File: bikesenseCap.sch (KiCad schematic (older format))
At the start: 43 parts

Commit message: Routing updated
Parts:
- removed D? (x4): LED_Small, symbol Device:LED_Small
- removed J? (x4): PAD, symbol cap1188:PAD
- removed R? (x4): 470, symbol Device:R_Small
- added D11: West, LEDs:LED_0805_HandSoldering, symbol Device:LED_Small
- added D12: NorthWest, LEDs:LED_0805_HandSoldering, symbol Device:LED_Small
- added D13: SouthWest, LEDs:LED_0805_HandSoldering, symbol Device:LED_Small
- added D14: North, LEDs:LED_0805_HandSoldering, symbol Device:LED_Small
- added D15: South, LEDs:LED_0805_HandSoldering, symbol Device:LED_Small
- added D16: NorthEast, LEDs:LED_0805_HandSoldering, symbol Device:LED_Small
- added D17: SouthEast, LEDs:LED_0805_HandSoldering, symbol Device:LED_Small
- added D18: East, LEDs:LED_0805_HandSoldering, symbol Device:LED_Small
- added R19, R21, R22, R27, R28, R31, R32, R35: 66, Resistors_SMD:R_0603_HandSoldering, symbol Device:R_Small
- added R20, R24, R25, R29, R30, R33, R34, R36: 100k, Resistors_SMD:R_0603_HandSoldering, symbol Device:R_Small
- added R23, R26: 10K, Resistors_SMD:R_0603_HandSoldering, symbol Device:R_Small
- added U3: TCA9534, digikey-footprints:SOIC-16_W7.5mm, symbol Interface_Expansion:TCA9534
- D1, D2: renamed from D?; footprint Diode_THT:D_DO-35_SOD27_P7.62mm_Horizontal -> Diodes_SMD:D_SOD-123
- D3, D4, D5, D6: renamed from D?; footprint (none) -> LEDs:LED_0603_HandSoldering
- J1: renamed from J?; footprint (none) -> SeeedOPL-Connector-2016:HW4-2.0
- J10, J11: renamed from J?; footprint (none) -> Connectors:1X01
- J2, J3, J4, J5: renamed from J?; footprint (none) -> capSensingStuff:SensePad
- JP1: renamed from JP?; footprint (none) -> Jumpers:SMT-JUMPER_2_NO_SILK
- R1, R10, R11, R12, R13, R14, R2, R3, R4, R5, R6, R7, R8, R9: renamed from R?; footprint (none) -> Resistors_SMD:R_0603_HandSoldering
- TH1: renamed from TH?; footprint (none) -> Resistors_SMD:R_0603_HandSoldering
- U1: renamed from U?; footprint (none) -> digikey-footprints:VOC_Sensor_LGA-10-1EP-2.7x4mm_CCS811B
- U2: renamed from U?; footprint (none) -> Housings_DFN_QFN:QFN-24_4x4mm_Pitch0.5mm_NoMask
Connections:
- net labels added: East, North, NorthEast, NorthWest, South, SouthEast, SouthWest, West
- wire segments 104 -> 192
- no-connect marks 3 -> 12
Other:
- note added: "CAP1188 - Cap Sensing Controller"
- note added: "CSS811 - VOC Sensor"
- note added: "I2C Connector"
- note added: "LED Interface"
- note added: "Power Flags"
- note added: "TCA9534 - IO Extender"

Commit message: up to revB
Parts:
- D11, D12, D13, D14, D15, D16, D17, D18: footprint LEDs:LED_0805_HandSoldering -> revLed:LED_1206_3216Metric_ReverseMount_Hole1.8x2.4mm
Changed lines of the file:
@@
 F 0 "D18" V 8646 2182 50  0000 R CNN
 F 1 "East" V 8555 2182 50  0000 R CNN
-F 2 "LEDs:LED_0805_HandSoldering" V 8600 2250 50  0001 C CNN
+F 2 "revLed:LED_1206_3216Metric_ReverseMount_Hole1.8x2.4mm" V 8600 2250 50  0001 C CNN
 F 3 "~" V 8600 2250 50  0001 C CNN
 	1    8600 2250
@@
 F 0 "D14" V 7525 1275 50  0000 R CNN
 F 1 "North" V 7425 1325 50  0000 R CNN
-F 2 "LEDs:LED_0805_HandSoldering" V 7500 1350 50  0001 C CNN
+F 2 "revLed:LED_1206_3216Metric_ReverseMount_Hole1.8x2.4mm" V 7500 1350 50  0001 C CNN
 F 3 "~" V 7500 1350 50  0001 C CNN
 	1    7500 1350
@@
 F 0 "D16" V 8146 1707 50  0000 R CNN
 F 1 "NorthEast" V 8055 1707 50  0000 R CNN
-F 2 "LEDs:LED_0805_HandSoldering" V 8100 1775 50  0001 C CNN
+F 2 "revLed:LED_1206_3216Metric_ReverseMount_Hole1.8x2.4mm" V 8100 1775 50  0001 C CNN
 F 3 "~" V 8100 1775 50  0001 C CNN
 	1    8100 1775
@@
 F 0 "D17" V 8146 2707 50  0000 R CNN
 F 1 "SouthEast" V 8055 2707 50  0000 R CNN
-F 2 "LEDs:LED_0805_HandSoldering" V 8100 2775 50  0001 C CNN
+F 2 "revLed:LED_1206_3216Metric_ReverseMount_Hole1.8x2.4mm" V 8100 2775 50  0001 C CNN
 F 3 "~" V 8100 2775 50  0001 C CNN
 	1    8100 2775
@@
 F 0 "D15" V 7546 3082 50  0000 R CNN
 F 1 "South" V 7455 3082 50  0000 R CNN
-F 2 "LEDs:LED_0805_HandSoldering" V 7500 3150 50  0001 C CNN
+F 2 "revLed:LED_1206_3216Metric_ReverseMount_Hole1.8x2.4mm" V 7500 3150 50  0001 C CNN
 F 3 "~" V 7500 3150 50  0001 C CNN
 	1    7500 3150
@@
 F 0 "D13" V 6996 2732 50  0000 R CNN
 F 1 "SouthWest" V 6875 2775 50  0000 R CNN
-F 2 "LEDs:LED_0805_HandSoldering" V 6950 2800 50  0001 C CNN
+F 2 "revLed:LED_1206_3216Metric_ReverseMount_Hole1.8x2.4mm" V 6950 2800 50  0001 C CNN
 F 3 "~" V 6950 2800 50  0001 C CNN
 	1    6950 2800
@@
 F 0 "D11" V 6471 2257 50  0000 R CNN
 F 1 "West" V 6380 2257 50  0000 R CNN
-F 2 "LEDs:LED_0805_HandSoldering" V 6425 2325 50  0001 C CNN
+F 2 "revLed:LED_1206_3216Metric_ReverseMount_Hole1.8x2.4mm" V 6425 2325 50  0001 C CNN
 F 3 "~" V 6425 2325 50  0001 C CNN
 	1    6425 2325
@@
 F 0 "D12" V 6996 1682 50  0000 R CNN
 F 1 "NorthWest" V 6875 1750 50  0000 R CNN
-F 2 "LEDs:LED_0805_HandSoldering" V 6950 1750 50  0001 C CNN
+F 2 "revLed:LED_1206_3216Metric_ReverseMount_Hole1.8x2.4mm" V 6950 1750 50  0001 C CNN
 F 3 "~" V 6950 1750 50  0001 C CNN
 	1    6950 1750

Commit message: REV C
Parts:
- removed D1, D2: 1N4148, Diodes_SMD:D_SOD-123, symbol Diode:1N4148
- removed J10, J11: Conn_01x01, Connectors:1X01, symbol Connector_Generic:Conn_01x01
- removed JP1: SolderJumper_2_Bridged, Jumpers:SMT-JUMPER_2_NO_SILK, symbol Jumper:SolderJumper_2_Bridged
- removed R9: 100K, Resistors_SMD:R_0603_HandSoldering, symbol Device:R_Small
- added R9: 10K, Resistors_SMD:R_0603_HandSoldering, symbol bikesenseCap-rescue:R_Small-Device
- D11, D12, D13, D14, D15, D16, D17, D18, D3, D4, D5, D6: symbol Device:LED_Small -> bikesenseCap-rescue:LED_Small-Device
- J1: symbol Connector:Conn_01x04_Male -> bikesenseCap-rescue:Conn_01x04_Male-Connector
- J2, J3, J4, J5: symbol cap1188:PAD -> bikesenseCap-rescue:PAD-cap1188
- R1, R10, R11, R12, R13, R14, R19, R2, R20, R21, R22, R23, R24, R25, R26, R27, R28, R29, R3, R30, R31, R32, R33, R34, R35, R36, R4, R5, R6, R7, R8: symbol Device:R_Small -> bikesenseCap-rescue:R_Small-Device
- TH1: symbol Device:Thermistor_NTC -> bikesenseCap-rescue:Thermistor_NTC-Device
- U1: symbol ccs811:CCS811 -> bikesenseCap-rescue:CCS811-ccs811
- U2: symbol cap1188:cap1188 -> bikesenseCap-rescue:cap1188-cap1188
- U3: symbol Interface_Expansion:TCA9534 -> bikesenseCap-rescue:TCA9534-Interface_Expansion
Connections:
- wire segments 192 -> 190

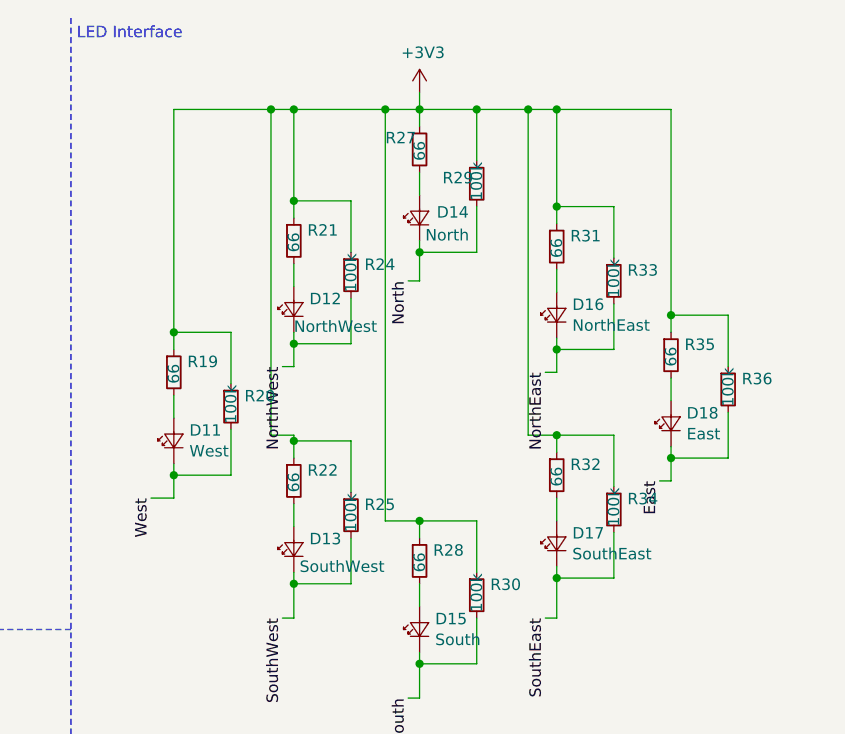
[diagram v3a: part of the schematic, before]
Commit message: REV C
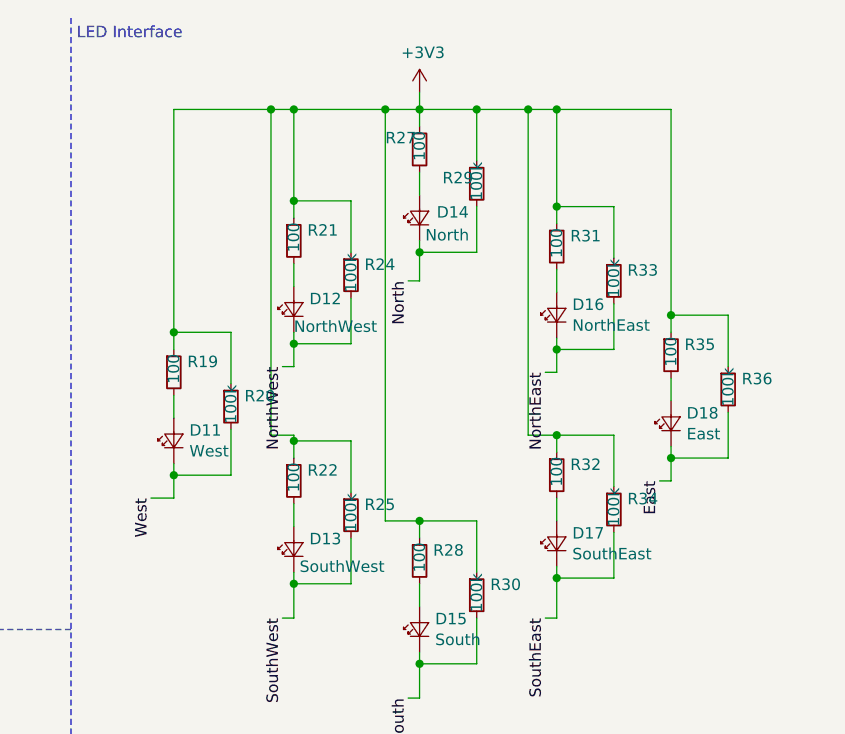
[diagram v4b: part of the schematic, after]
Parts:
- J1: Arrow# (none) -> 110990037
- R19, R21, R22, R27, R28, R31, R32, R35: value 66 -> 100
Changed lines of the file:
@@
 F 1 "Conn_01x04_Male" H 1050 825 50  0000 C CNN
 F 2 "SeeedOPL-Connector-2016:HW4-2.0" H 1000 1100 50  0001 C CNN
-F 3 "~" H 1000 1100 50  0001 C CNN
+F 3 "https://www.arrow.com/en/products/110990037/seeed-technology-limited" H 1000 1100 50  0001 C CNN
+F 4 "110990037" H 1000 1100 50  0001 C CNN "Arrow#"
 	1    1000 1100
 	1    0    0    -1
@@
 P 8600 1950
 F 0 "R35" H 8659 1996 50  0000 L CNN
-F 1 "66" V 8600 1900 50  0000 L CNN
+F 1 "100" V 8600 1900 50  0000 L CNN
 F 2 "Resistors_SMD:R_0603_HandSoldering" H 8600 1950 50  0001 C CNN
 F 3 "~" H 8600 1950 50  0001 C CNN
@@
 P 7500 1050
 F 0 "R27" H 7350 1100 50  0000 L CNN
-F 1 "66" V 7500 1000 50  0000 L CNN
+F 1 "100" V 7500 1000 50  0000 L CNN
 F 2 "Resistors_SMD:R_0603_HandSoldering" H 7500 1050 50  0001 C CNN
 F 3 "~" H 7500 1050 50  0001 C CNN
@@
 P 8100 1475
 F 0 "R31" H 8159 1521 50  0000 L CNN
-F 1 "66" V 8100 1425 50  0000 L CNN
+F 1 "100" V 8100 1425 50  0000 L CNN
 F 2 "Resistors_SMD:R_0603_HandSoldering" H 8100 1475 50  0001 C CNN
 F 3 "~" H 8100 1475 50  0001 C CNN
@@
 P 8100 2475
 F 0 "R32" H 8159 2521 50  0000 L CNN
-F 1 "66" V 8100 2425 50  0000 L CNN
+F 1 "100" V 8100 2425 50  0000 L CNN
 F 2 "Resistors_SMD:R_0603_HandSoldering" H 8100 2475 50  0001 C CNN
 F 3 "~" H 8100 2475 50  0001 C CNN
@@
 P 7500 2850
 F 0 "R28" H 7559 2896 50  0000 L CNN
-F 1 "66" V 7500 2800 50  0000 L CNN
+F 1 "100" V 7500 2800 50  0000 L CNN
 F 2 "Resistors_SMD:R_0603_HandSoldering" H 7500 2850 50  0001 C CNN
 F 3 "~" H 7500 2850 50  0001 C CNN
@@
 P 6950 2500
 F 0 "R22" H 7009 2546 50  0000 L CNN
-F 1 "66" V 6950 2450 50  0000 L CNN
+F 1 "100" V 6950 2450 50  0000 L CNN
 F 2 "Resistors_SMD:R_0603_HandSoldering" H 6950 2500 50  0001 C CNN
 F 3 "~" H 6950 2500 50  0001 C CNN
@@
 P 6425 2025
 F 0 "R19" H 6484 2071 50  0000 L CNN
-F 1 "66" V 6425 1975 50  0000 L CNN
+F 1 "100" V 6425 1975 50  0000 L CNN
 F 2 "Resistors_SMD:R_0603_HandSoldering" H 6425 2025 50  0001 C CNN
 F 3 "~" H 6425 2025 50  0001 C CNN
@@
 P 6950 1450
 F 0 "R21" H 7009 1496 50  0000 L CNN
-F 1 "66" V 6950 1400 50  0000 L CNN
+F 1 "100" V 6950 1400 50  0000 L CNN
 F 2 "Resistors_SMD:R_0603_HandSoldering" H 6950 1450 50  0001 C CNN
 F 3 "~" H 6950 1450 50  0001 C CNN

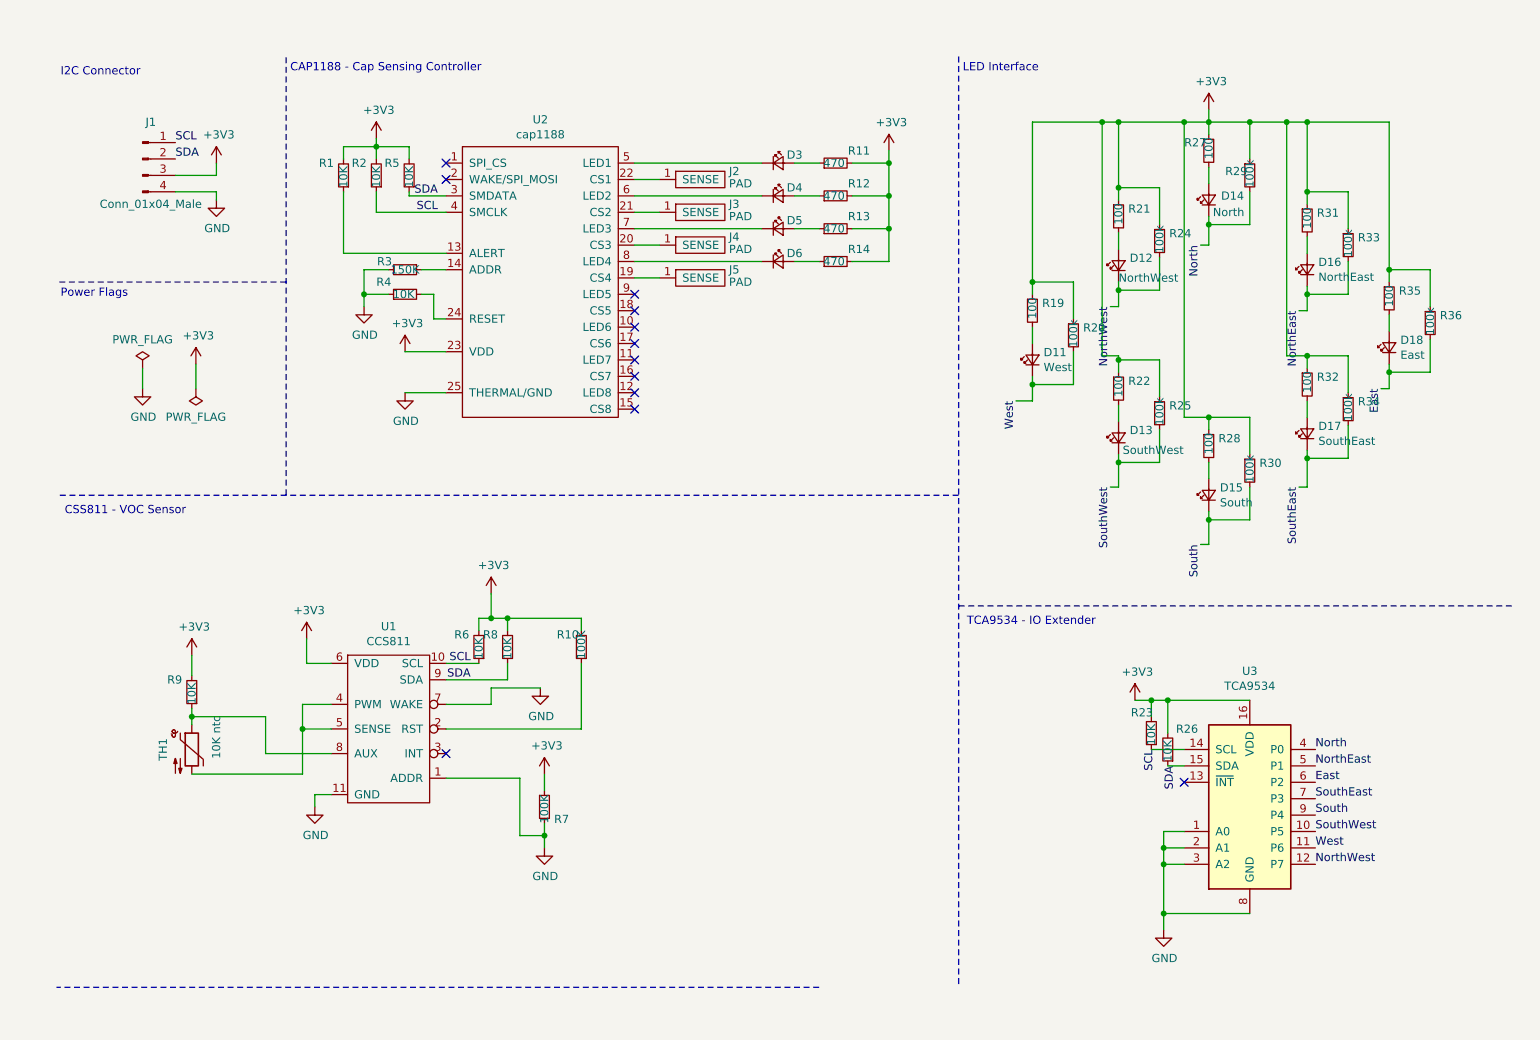
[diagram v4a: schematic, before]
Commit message: update
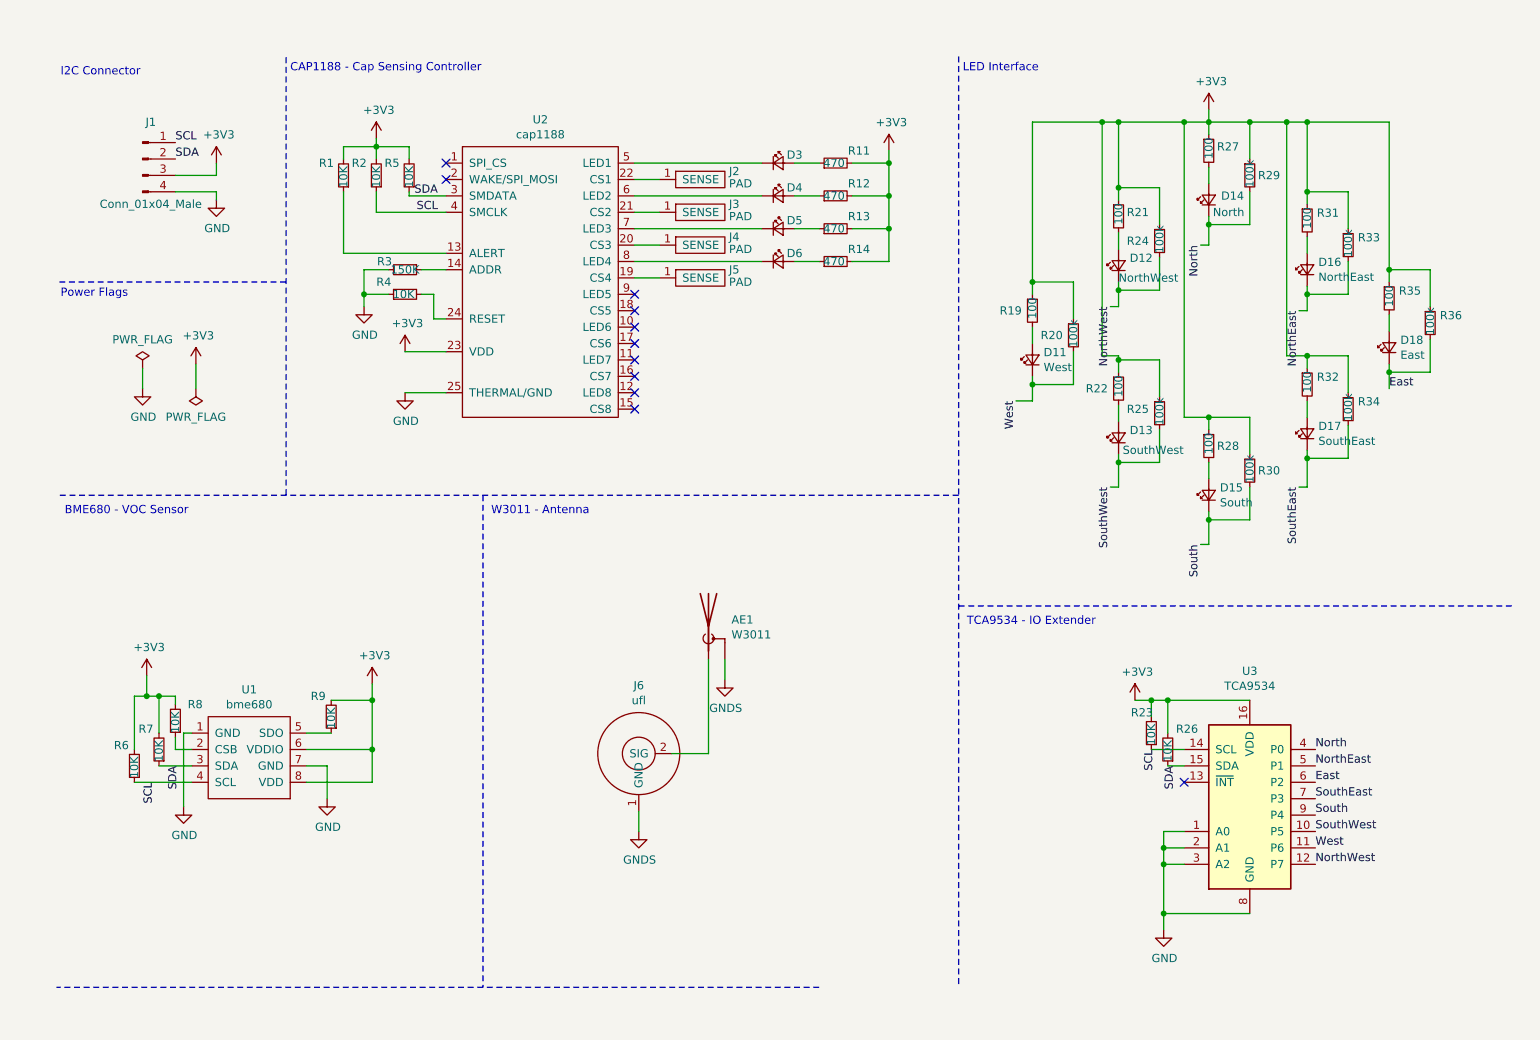
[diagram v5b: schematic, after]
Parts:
- removed R10: 100K, Resistors_SMD:R_0603_HandSoldering, symbol bikesenseCap-rescue:R_Small-Device
- removed TH1: 10K ntc, Resistors_SMD:R_0603_HandSoldering, symbol bikesenseCap-rescue:Thermistor_NTC-Device
- removed U1: CCS811, digikey-footprints:VOC_Sensor_LGA-10-1EP-2.7x4mm_CCS811B, symbol bikesenseCap-rescue:CCS811-ccs811
- added AE1: W3011, antenna:w3011, symbol Device:Antenna_Shield
- added J6: ufl, .pretty:ufl, symbol ufl:ufl
- added U1: bme680, kicad-libraries:BME680, symbol bme680:bme680
- R7: value 100K -> 10K
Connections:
- net +3V3: now also R7.2, U1.6 (VDDIO), U1.8 (VDD); no longer R7.1
- net GND: now also U1.1 (GND), U1.7 (GND); no longer R7.2
- net SCL: now also U1.4 (SCL)
- net SDA: now also R7.1, U1.3 (SDA); no longer R8.1
- net at R9.1: now also U1.5 (SDO)
- new net: R8.1, U1.2 (CSB)
- new net: AE1.1 (A), J6.2 (SIG)
- new net GNDS: AE1.2 (Shield), J6.1 (GND)
- no-connect marks 12 -> 11
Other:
- note added: "BME680 - VOC Sensor"
- note added: "W3011 - Antenna"
- note removed: "CSS811 - VOC Sensor"
